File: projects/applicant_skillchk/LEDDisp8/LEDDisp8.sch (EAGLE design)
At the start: 26 parts, among them J1 4X2, J2 3X1A

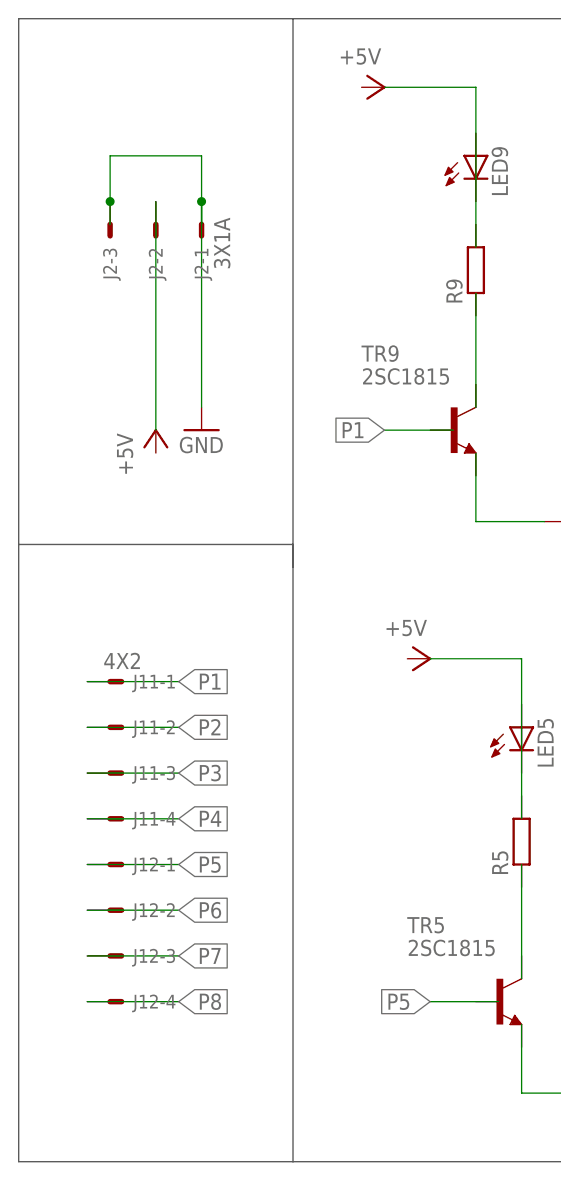
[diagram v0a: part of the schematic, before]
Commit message: 回路図作成
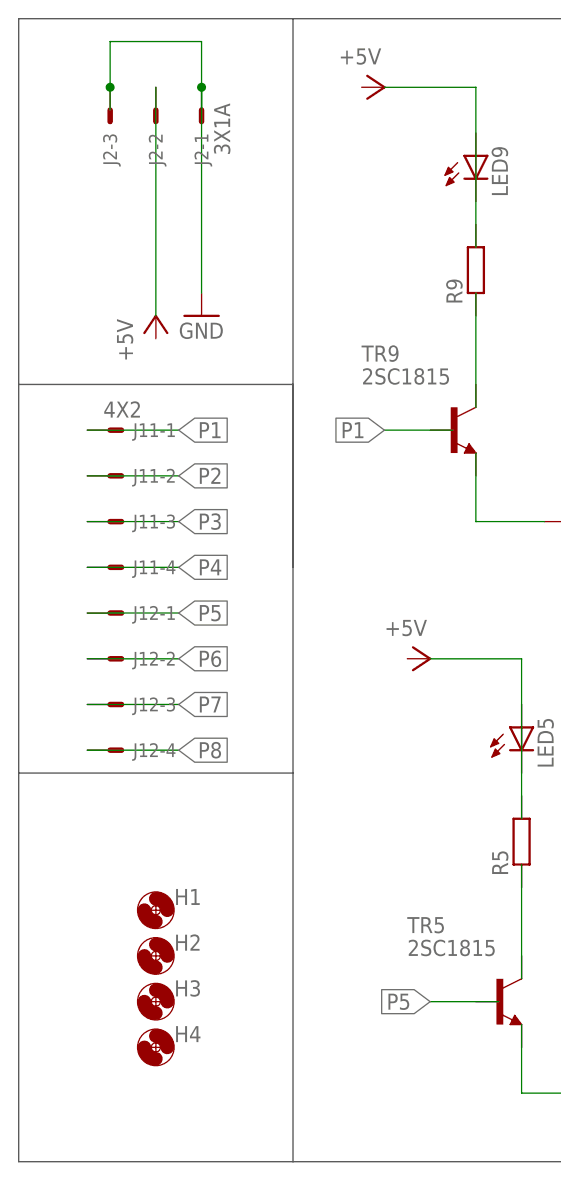
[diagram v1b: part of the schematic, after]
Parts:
- added H1, H2, H3, H4: HOLE3.3M3BOLT, Hole:HOLE3.3M3BOLT
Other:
- moved on the sheet: J11-1, J11-2, J11-3, J11-4, J12-1, J12-2, J12-3, J12-4, J2-1, J2-2, J2-3
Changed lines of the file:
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@@
 <part name="GND9" library="supply1" deviceset="GND" device=""/>
 <part name="P+9" library="supply1" deviceset="+5V" device=""/>
+<part name="H1" library="Hole" deviceset="HOLE3.3" device="M3BOLT"/>
+<part name="H2" library="Hole" deviceset="HOLE3.3" device="M3BOLT"/>
+<part name="H3" library="Hole" deviceset="HOLE3.3" device="M3BOLT"/>
+<part name="H4" library="Hole" deviceset="HOLE3.3" device="M3BOLT"/>
 </parts>
 <sheets>
 <sheet>
 <plain>
-<wire x1="-40.64" y1="104.14" x2="-40.64" y2="45.72" width="0.1524" layer="97"/>
-<wire x1="-40.64" y1="45.72" x2="-40.64" y2="-22.86" width="0.1524" layer="97"/>
+<wire x1="-40.64" y1="104.14" x2="-40.64" y2="63.5" width="0.1524" layer="97"/>
+<wire x1="-40.64" y1="63.5" x2="-40.64" y2="20.32" width="0.1524" layer="97"/>
+<wire x1="-40.64" y1="20.32" x2="-40.64" y2="-22.86" width="0.1524" layer="97"/>
 <wire x1="-40.64" y1="-22.86" x2="-10.16" y2="-22.86" width="0.1524" layer="97"/>
 <wire x1="-10.16" y1="-22.86" x2="137.16" y2="-22.86" width="0.1524" layer="97"/>
@@
 <wire x1="137.16" y1="104.14" x2="-10.16" y2="104.14" width="0.1524" layer="97"/>
 <wire x1="-10.16" y1="104.14" x2="-40.64" y2="104.14" width="0.1524" layer="97"/>
-<wire x1="-40.64" y1="45.72" x2="-10.16" y2="45.72" width="0.1524" layer="97"/>
-<wire x1="-10.16" y1="45.72" x2="-10.16" y2="43.18" width="0.1524" layer="97"/>
-<wire x1="-10.16" y1="43.18" x2="-10.16" y2="-22.86" width="0.1524" layer="97"/>
-<wire x1="-10.16" y1="43.18" x2="-10.16" y2="104.14" width="0.1524" layer="97"/>
+<wire x1="-40.64" y1="63.5" x2="-10.16" y2="63.5" width="0.1524" layer="97"/>
+<wire x1="-10.16" y1="63.5" x2="-10.16" y2="43.18" width="0.1524" layer="97"/>
+<wire x1="-10.16" y1="43.18" x2="-10.16" y2="20.32" width="0.1524" layer="97"/>
+<wire x1="-10.16" y1="20.32" x2="-10.16" y2="-22.86" width="0.1524" layer="97"/>
+<wire x1="-10.16" y1="43.18" x2="-10.16" y2="63.5" width="0.1524" layer="97"/>
+<wire x1="-10.16" y1="63.5" x2="-10.16" y2="104.14" width="0.1524" layer="97"/>
+<wire x1="-40.64" y1="20.32" x2="-10.16" y2="20.32" width="0.1524" layer="97"/>
 </plain>
 <instances>
-<instance part="J1" gate="1-1" x="-27.94" y="30.48"/>
-<instance part="J1" gate="1-3" x="-27.94" y="20.32"/>
-<instance part="J1" gate="1-2" x="-27.94" y="25.4"/>
-<instance part="J1" gate="1-4" x="-27.94" y="15.24"/>
-<instance part="J1" gate="2-1" x="-27.94" y="10.16"/>
-<instance part="J1" gate="2-2" x="-27.94" y="5.08"/>
-<instance part="J1" gate="2-3" x="-27.94" y="0"/>
-<instance part="J1" gate="2-4" x="-27.94" y="-5.08"/>
-<instance part="J2" gate="-1" x="-20.32" y="78.74" rot="R270"/>
-<instance part="J2" gate="-2" x="-25.4" y="78.74" rot="R270"/>
-<instance part="J2" gate="-3" x="-30.48" y="78.74" rot="R270"/>
+<instance part="J1" gate="1-1" x="-27.94" y="58.42"/>
+<instance part="J1" gate="1-3" x="-27.94" y="48.26"/>
+<instance part="J1" gate="1-2" x="-27.94" y="53.34"/>
+<instance part="J1" gate="1-4" x="-27.94" y="43.18"/>
+<instance part="J1" gate="2-1" x="-27.94" y="38.1"/>
+<instance part="J1" gate="2-2" x="-27.94" y="33.02"/>
+<instance part="J1" gate="2-3" x="-27.94" y="27.94"/>
+<instance part="J1" gate="2-4" x="-27.94" y="22.86"/>
+<instance part="J2" gate="-1" x="-20.32" y="91.44" rot="R270"/>
+<instance part="J2" gate="-2" x="-25.4" y="91.44" rot="R270"/>
+<instance part="J2" gate="-3" x="-30.48" y="91.44" rot="R270"/>
 <instance part="R1" gate="G$1" x="43.18" y="76.2" rot="R90"/>
 <instance part="LED1" gate="G$1" x="43.18" y="88.9"/>
 <instance part="TR1" gate="G$1" x="40.64" y="58.42"/>
-<instance part="P+1" gate="1" x="-25.4" y="58.42"/>
-<instance part="GND1" gate="1" x="-20.32" y="58.42"/>
+<instance part="P+1" gate="1" x="-25.4" y="71.12"/>
+<instance part="GND1" gate="1" x="-20.32" y="71.12"/>
 <instance part="GND7" gate="1" x="53.34" y="48.26" rot="R90"/>
 <instance part="P+2" gate="1" x="33.02" y="96.52" rot="R270"/>
@@
 <instance part="GND9" gate="1" x="129.54" y="-17.78" rot="R90"/>
 <instance part="P+9" gate="1" x="109.22" y="30.48" rot="R270"/>
+<instance part="H1" gate="G$1" x="-25.4" y="5.08"/>
+<instance part="H2" gate="G$1" x="-25.4" y="0"/>
+<instance part="H3" gate="G$1" x="-25.4" y="-5.08"/>
+<instance part="H4" gate="G$1" x="-25.4" y="-10.16"/>
 </instances>
 <busses>
@@
 <segment>
 <pinref part="J2" gate="-2" pin="S"/>
-<wire x1="-25.4" y1="83.82" x2="-25.4" y2="58.42" width="0.1524" layer="91"/>
+<wire x1="-25.4" y1="96.52" x2="-25.4" y2="71.12" width="0.1524" layer="91"/>
 </segment>
 </net>
 <net name="GND" class="0">
 <segment>
-<wire x1="-30.48" y1="81.28" x2="-30.48" y2="83.82" width="0.1524" layer="91"/>
-<wire x1="-30.48" y1="83.82" x2="-30.48" y2="88.9" width="0.1524" layer="91"/>
-<wire x1="-30.48" y1="88.9" x2="-20.32" y2="88.9" width="0.1524" layer="91"/>
-<wire x1="-20.32" y1="88.9" x2="-20.32" y2="83.82" width="0.1524" layer="91"/>
+<wire x1="-30.48" y1="93.98" x2="-30.48" y2="96.52" width="0.1524" layer="91"/>
+<wire x1="-30.48" y1="96.52" x2="-30.48" y2="101.6" width="0.1524" layer="91"/>
+<wire x1="-30.48" y1="101.6" x2="-20.32" y2="101.6" width="0.1524" layer="91"/>
+<wire x1="-20.32" y1="101.6" x2="-20.32" y2="96.52" width="0.1524" layer="91"/>
 <pinref part="GND1" gate="1" pin="GND"/>
-<wire x1="-20.32" y1="83.82" x2="-20.32" y2="81.28" width="0.1524" layer="91"/>
-<wire x1="-20.32" y1="60.96" x2="-20.32" y2="83.82" width="0.1524" layer="91"/>
-<junction x="-20.32" y="83.82"/>
+<wire x1="-20.32" y1="96.52" x2="-20.32" y2="93.98" width="0.1524" layer="91"/>
+<wire x1="-20.32" y1="73.66" x2="-20.32" y2="96.52" width="0.1524" layer="91"/>
+<junction x="-20.32" y="96.52"/>
 <pinref part="J2" gate="-1" pin="S"/>
 <pinref part="J2" gate="-3" pin="S"/>
-<junction x="-30.48" y="83.82"/>
+<junction x="-30.48" y="96.52"/>
 </segment>
 <segment>
@@
 <segment>
 <pinref part="J1" gate="1-1" pin="S"/>
-<wire x1="-33.02" y1="30.48" x2="-22.86" y2="30.48" width="0.1524" layer="91"/>
-<label x="-22.86" y="30.48" size="1.778" layer="95" xref="yes"/>
+<wire x1="-33.02" y1="58.42" x2="-22.86" y2="58.42" width="0.1524" layer="91"/>
+<label x="-22.86" y="58.42" size="1.778" layer="95" xref="yes"/>
 </segment>
 <segment>
@@
 <segment>
 <pinref part="J1" gate="1-2" pin="S"/>
-<wire x1="-33.02" y1="25.4" x2="-22.86" y2="25.4" width="0.1524" layer="91"/>
-<label x="-22.86" y="25.4" size="1.778" layer="95" xref="yes"/>
+<wire x1="-33.02" y1="53.34" x2="-22.86" y2="53.34" width="0.1524" layer="91"/>
+<label x="-22.86" y="53.34" size="1.778" layer="95" xref="yes"/>
 </segment>
 <segment>
@@
 <segment>
 <pinref part="J1" gate="1-3" pin="S"/>
-<wire x1="-33.02" y1="20.32" x2="-22.86" y2="20.32" width="0.1524" layer="91"/>
-<label x="-22.86" y="20.32" size="1.778" layer="95" xref="yes"/>
+<wire x1="-33.02" y1="48.26" x2="-22.86" y2="48.26" width="0.1524" layer="91"/>
+<label x="-22.86" y="48.26" size="1.778" layer="95" xref="yes"/>
 </segment>
 <segment>
@@
 <segment>
 <pinref part="J1" gate="1-4" pin="S"/>
-<wire x1="-33.02" y1="15.24" x2="-22.86" y2="15.24" width="0.1524" layer="91"/>
-<label x="-22.86" y="15.24" size="1.778" layer="95" xref="yes"/>
+<wire x1="-33.02" y1="43.18" x2="-22.86" y2="43.18" width="0.1524" layer="91"/>
+<label x="-22.86" y="43.18" size="1.778" layer="95" xref="yes"/>
 </segment>
 <segment>
@@
 <segment>
 <pinref part="J1" gate="2-1" pin="S"/>
-<wire x1="-33.02" y1="10.16" x2="-22.86" y2="10.16" width="0.1524" layer="91"/>
-<label x="-22.86" y="10.16" size="1.778" layer="95" xref="yes"/>
+<wire x1="-33.02" y1="38.1" x2="-22.86" y2="38.1" width="0.1524" layer="91"/>
+<label x="-22.86" y="38.1" size="1.778" layer="95" xref="yes"/>
 </segment>
 <segment>
@@
 <segment>
 <pinref part="J1" gate="2-2" pin="S"/>
-<wire x1="-33.02" y1="5.08" x2="-22.86" y2="5.08" width="0.1524" layer="91"/>
-<label x="-22.86" y="5.08" size="1.778" layer="95" xref="yes"/>
+<wire x1="-33.02" y1="33.02" x2="-22.86" y2="33.02" width="0.1524" layer="91"/>
+<label x="-22.86" y="33.02" size="1.778" layer="95" xref="yes"/>
 </segment>
 <segment>
@@
 <segment>
 <pinref part="J1" gate="2-3" pin="S"/>
-<wire x1="-33.02" y1="0" x2="-22.86" y2="0" width="0.1524" layer="91"/>
-<label x="-22.86" y="0" size="1.778" layer="95" xref="yes"/>
+<wire x1="-33.02" y1="27.94" x2="-22.86" y2="27.94" width="0.1524" layer="91"/>
+<label x="-22.86" y="27.94" size="1.778" layer="95" xref="yes"/>
 </segment>
 <segment>
@@
 <segment>
 <pinref part="J1" gate="2-4" pin="S"/>
-<wire x1="-33.02" y1="-5.08" x2="-22.86" y2="-5.08" width="0.1524" layer="91"/>
-<label x="-22.86" y="-5.08" size="1.778" layer="95" xref="yes"/>
-</segment>
-<segment>
+<wire x1="-33.02" y1="22.86" x2="-22.86" y2="22.86" width="0.1524" layer="91"/>
+<label x="-22.86" y="22.86" size="1.778" layer="95" xref="yes"/>
+</segment>
+<segment>
